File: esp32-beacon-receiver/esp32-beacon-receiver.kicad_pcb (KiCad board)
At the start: 2 copper layers, 64 x 46 mm, 67 parts, among them J1 USB_B_Micro, J2 Micro_SD_Card, J3 Neopixel, J4 Conn_02x05_Odd_Even, M1 Motor_Servo, Q1 Q_PMOS_GSD, Q2 Q_PMOS_GSD, Q3 MMBT3904, Q4 MMBT3904, U1 PCF8563T, U2 CH340C, U3 ESP32-WROOM-32, U4 TPS54331, U5 FP6291, U6 MAX98357, U7 Logo, Y1 Crystal

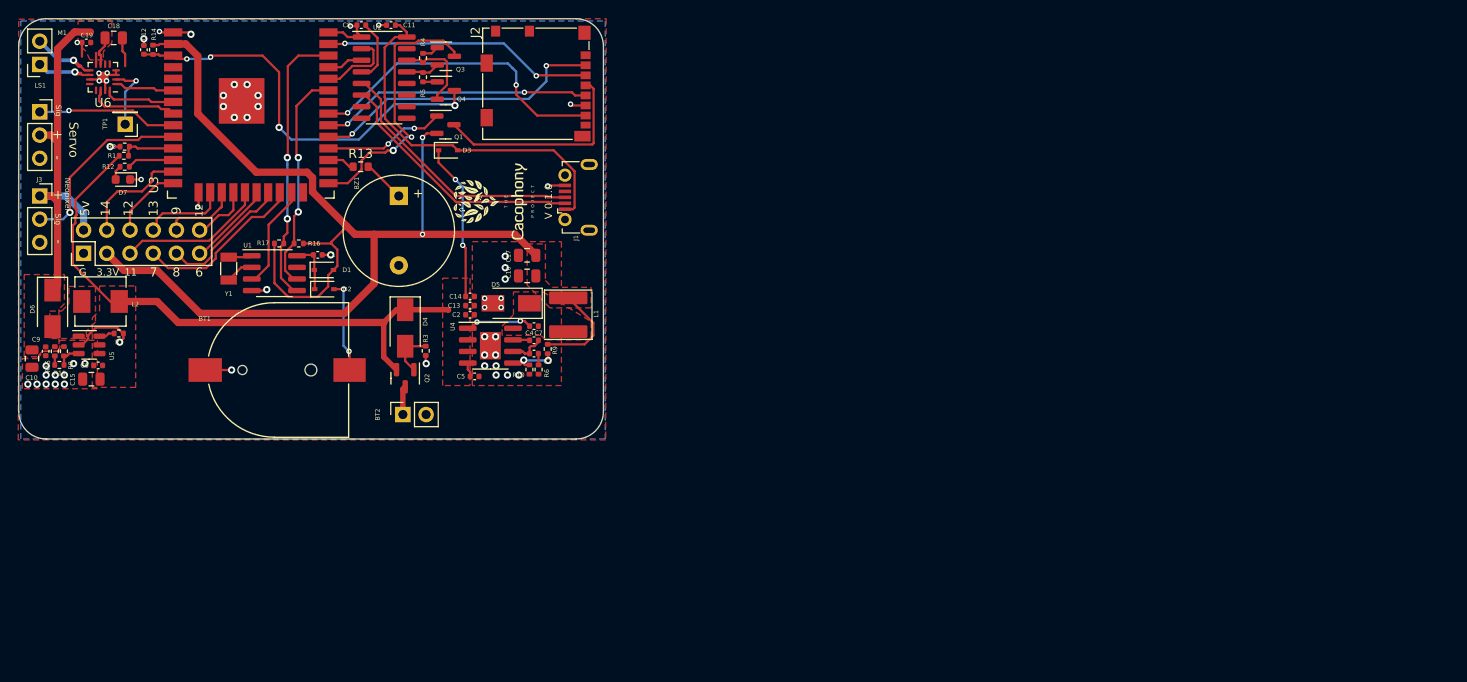
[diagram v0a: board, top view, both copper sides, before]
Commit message: Fixed some things
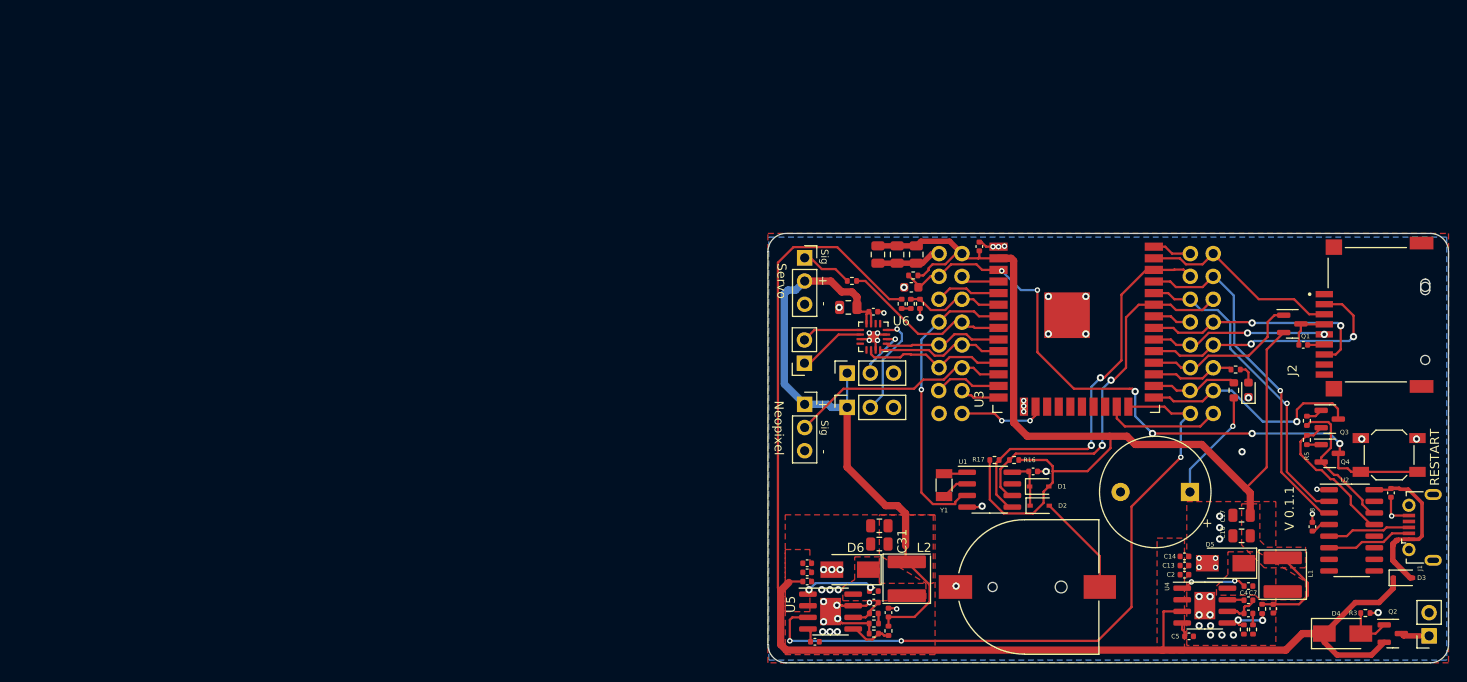
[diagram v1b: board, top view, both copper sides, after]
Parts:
- removed TP1: TestPoint, Connector_PinHeader_2.54mm:PinHeader_1x01_P2.54mm_Vertical
- added C20: 47pF, Capacitor_SMD:C_0402_1005Metric, F.Cu at (159.6, 91.9)
- added C21: 10nF, Capacitor_SMD:C_0402_1005Metric, F.Cu at (152.3, 89.6)
- added C22: 22uF, Capacitor_SMD:C_0805_2012Metric, F.Cu at (164.2, 53.8)
- added C23: 10nF, Capacitor_SMD:C_0402_1005Metric, F.Cu at (153.2, 96.2)
- added C24: 22uF, Capacitor_SMD:C_0805_2012Metric, F.Cu at (160.0, 53.8)
- added C25: 22uF, Capacitor_SMD:C_0805_2012Metric, F.Cu at (162.1, 53.8)
- added C26: 1uF, Capacitor_SMD:C_0402_1005Metric, F.Cu at (171.1, 52.9)
- added C27: 100nF, Capacitor_SMD:C_0402_1005Metric, F.Cu at (159.6, 90.7)
- added C28: 10uF, Capacitor_SMD:C_0603_1608Metric, F.Cu at (163.7, 57.4)
- added C29: 1uF, Capacitor_SMD:C_0402_1005Metric, F.Cu at (161.2, 93.0)
- added C30: 22uF, Capacitor_SMD:C_0805_2012Metric, F.Cu at (160.2, 83.5)
- added C31: 22uF, Capacitor_SMD:C_0805_2012Metric, F.Cu at (160.2, 85.5)
- added J5: Conn_01x03, Connector_PinSocket_2.54mm:PinSocket_1x03_P2.54mm_Vertical, F.Cu at (156.7, 70.5)
- added R18: 10K, Resistor_SMD:R_0402_1005Metric, F.Cu at (157.2, 56.7)
- added SW2: SW_Push, Button_Switch_SMD:SW_SPST_SKQG_WithStem, F.Cu at (216.0, 75.8)
- C1, C6, C9: value 100nF -> 1uF
- C10, C15: value 22uF -> 4.7uF; footprint Capacitor_SMD:C_0805_2012Metric -> Capacitor_SMD:C_0402_1005Metric
- C12: value 100nF -> 1nF
- C16, C17: value 47uF -> 22uF
- J2: footprint cacophony-footprints:microSD_HC_Molex_104031-0811 -> cacophony-footprints:SD_Micro
- J4: value Conn_02x05_Odd_Even -> Conn_01x03; footprint Connector_PinHeader_2.54mm:PinHeader_2x06_P2.54mm_Vertical -> Connector_PinSocket_2.54mm:PinSocket_1x03_P2.54mm_Vertical
- L2: value 3.3uH -> 6.8uH; footprint Inductor_SMD:L_Sunlord_MWSA0518_5.4x5.2mm -> cacophony-footprints:SWPA5040S
- R11: value 68K -> 12K
- R15: value 22K -> 2.2K
- R7: value 10K -> 100K
- R8: value 12K -> 29.4k
- U5: value FP6291 -> TPS54331; footprint Package_TO_SOT_SMD:SOT-23-6 -> Package_SO:SOIC-8-1EP_3.9x4.9mm_P1.27mm_EP2.29x3mm
- U7: footprint cacophony-footprints:logo_small -> cacophony-footprints:logo; moved to B.Cu
- moved C9 137.3 mm to (203.3, 92.6)
- moved C6 131.9 mm to (206.6, 63.7), turned to 0 degrees
- moved D7 125.3 mm to (200.6, 68.6), turned to 90 degrees
- moved R12 123.6 mm to (199.2, 66.4), turned to 180 degrees
- moved C11 120.8 mm to (216.2, 79.9), turned to -90 degrees
- moved C8 117.7 mm to (207.6, 83.6), turned to 90 degrees
- moved U2 116.9 mm to (211.9, 84.0)
- moved BT2 114.9 mm to (220.4, 95.5), turned to 180 degrees
- moved D3 114.5 mm to (217.5, 89.2)
- moved Q2 111.7 mm to (216.4, 95.3), turned to 0 degrees
- moved D4 107.9 mm to (210.9, 95.3), turned to 0 degrees
- moved R3 106.8 mm to (213.4, 93.0), turned to 0 degrees
- moved Q3 104.6 mm to (209.5, 71.8)
- moved Q4 104.6 mm to (209.5, 75.6)
- moved R4 104.6 mm to (207.0, 72.0)
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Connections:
- net /CS renamed SD_CS
- net /IO0 renamed BOOT_MODE
- net /MISO renamed SD_MISO
- net /MOSI renamed SD_MOSI
- net /RXD0 renamed RXD0
- net /SCK renamed SD_SCK
- net /SCL renamed SCL
- net /SDA renamed SDA
- net /SD_ENABLE renamed SD_ENABLE
- net /TXD0 renamed TXD0
- C10 pad 1: +5V -> VCC
- C12 pad 1: /EN -> Net-(C12-Pad1)
- C12 pad 2: GND -> Net-(C12-Pad2)
- C6 pad 1: VCC -> Net-(C6-Pad1)
- C9 pad 1: +5V -> +3V3
- D6 pad 1: +5V -> Net-(C27-Pad2)
- D6 pad 2: Net-(D6-Pad2) -> GND
- J2 pad 4: Net-(J2-Pad4) -> Net-(C6-Pad1)
- J3 pad 2: /Neopixel -> Neopixel
- J4 pad 1: GND -> +5V
- J4 pad 2: +5V -> /GAIN
- J4 pad 3: +3V3 -> GND
- L2 pad 1: VCC -> Net-(C27-Pad2)
- L2 pad 2: Net-(D6-Pad2) -> +5V
- M1 pad 1: /SERVO -> Net-(M1-Pad1)
- Q1 pad 3: Net-(J2-Pad4) -> Net-(C6-Pad1)
- Q4 pad 3: /EN -> EN
- R1 pad 1: VCC -> Net-(R1-Pad1)
- R1 pad 2: /BATTERY_VOLTAGE -> BATTERY_VOLTAGE
- R11 pad 1: Net-(R11-Pad1) -> +5V
- R12 pad 2: /STATUS_LED -> STATUS_LED
- R13 pad 1: /BUZZER -> BUZZER
- R14 pad 2: /EN -> EN
- R15 pad 2: +5V -> GND
- R2 pad 1: /BATTERY_VOLTAGE -> BATTERY_VOLTAGE
- R7 pad 1: Net-(R7-Pad1) -> VCC
- R7 pad 2: GND -> Net-(R1-Pad1)
- R8 pad 1: Net-(R11-Pad1) -> Net-(C12-Pad2)
- U1 pad 3: /RTC_INT# -> ~{RTC_INT}
- U3 pad 10: /Neopixel -> I2S_BCLK
- U3 pad 11: /BATTERY_VOLTAGE -> I2S_LRCLK
- U3 pad 12: /STATUS_LED -> Neopixel
- U3 pad 13: /IO14 -> IO14/TMS
- U3 pad 14: /IO12 -> IO12/TDI
- U3 pad 16: /IO13 -> IO13TCK
- U3 pad 17: /IO9 -> unconnected-(U3-Pad17)
- U3 pad 18: /IO10 -> unconnected-(U3-Pad18)
- U3 pad 19: /IO11 -> unconnected-(U3-Pad19)
- U3 pad 20: /IO6 -> unconnected-(U3-Pad20)
- U3 pad 21: /IO8 -> unconnected-(U3-Pad21)
- U3 pad 22: /IO7 -> unconnected-(U3-Pad22)
- U3 pad 23: /RTC_INT# -> IO15/TDO
- U3 pad 24: unconnected-(U3-Pad24) -> 5V_ENABLE
- U3 pad 26: unconnected-(U3-Pad26) -> BUZZER
- U3 pad 27: /BUZZER -> STATUS_LED
- U3 pad 3: /EN -> EN
- U3 pad 6: /DIN -> BATTERY_VOLTAGE
- U3 pad 7: /BCLK -> ~{RTC_INT}
- U3 pad 8: /LRCLK -> SERVO
- U3 pad 9: /SERVO -> I2S_DOUT
- U5 pad 1: Net-(D6-Pad2) -> Net-(C27-Pad1)
- U5 pad 2: GND -> VCC
- U5 pad 3: Net-(R11-Pad1) -> 5V_ENABLE
- U5 pad 4: /5V_EN -> Net-(C23-Pad1)
- U5 pad 5: VCC -> Net-(R11-Pad2)
- U5 pad 6: Net-(R7-Pad1) -> Net-(C12-Pad1)
- U6 pad 1: /DIN -> I2S_DOUT
- U6 pad 14: /LRCLK -> I2S_LRCLK
- U6 pad 16: /BCLK -> I2S_BCLK
- U6 pad 2: Net-(TP1-Pad1) -> /GAIN
- U6 pad 4: GND -> SD_MODE
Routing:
- net 5V_ENABLE: track 0.00 -> 74.3 mm, vias 0 -> 3
- net EN: track 0.00 -> 74.2 mm, vias 0 -> 6
- net VCC: track 81.4 -> 147.6 mm, vias 2 -> 0
- net /EN: track 45.1 -> 0.00 mm, vias 4 -> 0
- net TXD0: track 3.94 -> 38.9 mm, vias 0 -> 1
- net ~{RTC_INT}: track 0.00 -> 32.7 mm, vias 0 -> 1
- net RXD0: track 8.45 -> 34.7 mm, vias 0 -> 1
- net Neopixel: track 0.00 -> 24.2 mm
- net Net-(J2-Pad4): track 23.2 -> 0.00 mm
- net Net-(C11-Pad1): track 41.0 -> 17.9 mm
- net +5V: track 47.4 -> 68.6 mm
- net /Neopixel: track 20.6 -> 0.00 mm, vias 1 -> 0
- net Net-(J1-Pad3): track 28.8 -> 9.14 mm
- net /IO7: track 18.9 -> 0.00 mm
- net Net-(J1-Pad2): track 28.2 -> 9.40 mm
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- added copper zone on F.Cu, net Net-(C27-Pad2)
- removed copper zone on F.Cu, net Net-(D6-Pad2)
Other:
- board size 64 x 46 mm -> 74.5 x 47 mm
- board text added: "+5V"
- board text added: "GAIN"
- board text added: "RESTART"
- board text added: "SD_MODE"
- board text added: "V 0.1.1"
- board text removed: "11"
- board text removed: "12"
- board text removed: "13"
- board text removed: "14"
- board text removed: "3.3V"
- board text removed: "5v"
- board text removed: "6"
- board text removed: "7"
- board text removed: "8"
- board text removed: "9"
- board text removed: "G"
- board text removed: "IO11"
- board text removed: "IO12"
- board text removed: "IO13"
- board text removed: "IO14"
- board text removed: "IO6"
- board text removed: "IO7"
- board text removed: "IO8"
- board text removed: "IO9"
- board text removed: "V 0.1.0"
